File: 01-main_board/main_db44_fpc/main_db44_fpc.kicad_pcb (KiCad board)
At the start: 4 copper layers, 65 x 26.5 mm, 4 parts, among them J1 DB44_Female

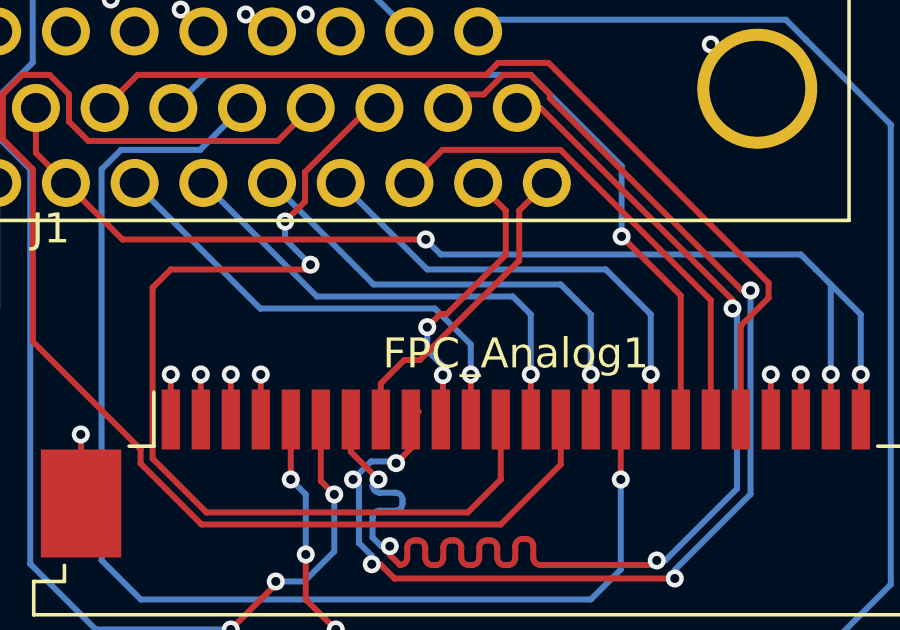
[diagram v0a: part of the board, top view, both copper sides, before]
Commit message: update db44
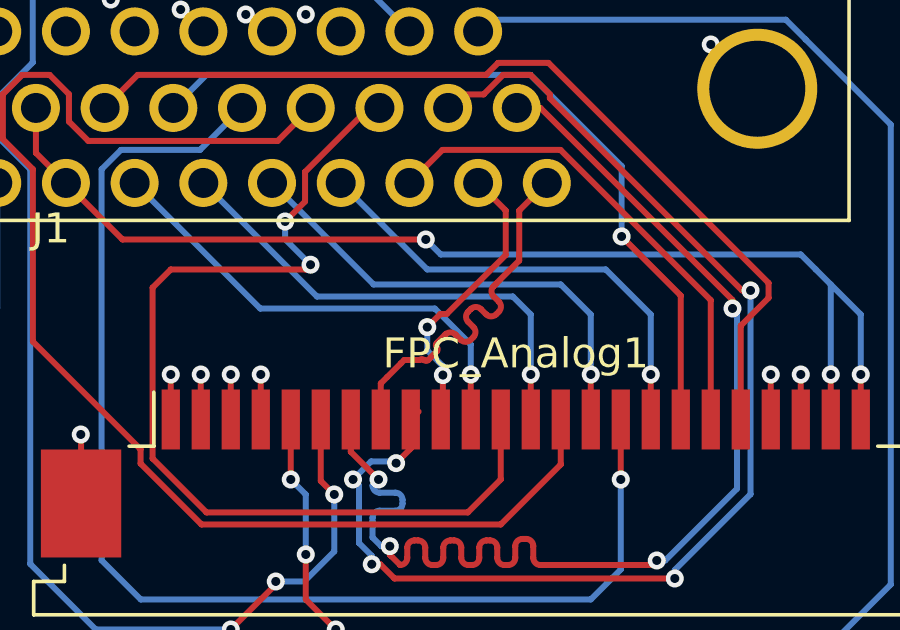
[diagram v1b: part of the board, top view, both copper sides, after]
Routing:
- net sg_sense_1_FL-: track 10.5 -> 12.7 mm
